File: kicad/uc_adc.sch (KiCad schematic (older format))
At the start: 13 parts, among them IC301 TPD4E001QDBV, IC302 TPD4E001QDBV, IC303 TPD4E001QDBV, IC304 TPD4E001QDBV, IC305 TPD4E001QDBV, IC306 TPD4E001QDBV, U301 TMS320F28388DZWTS

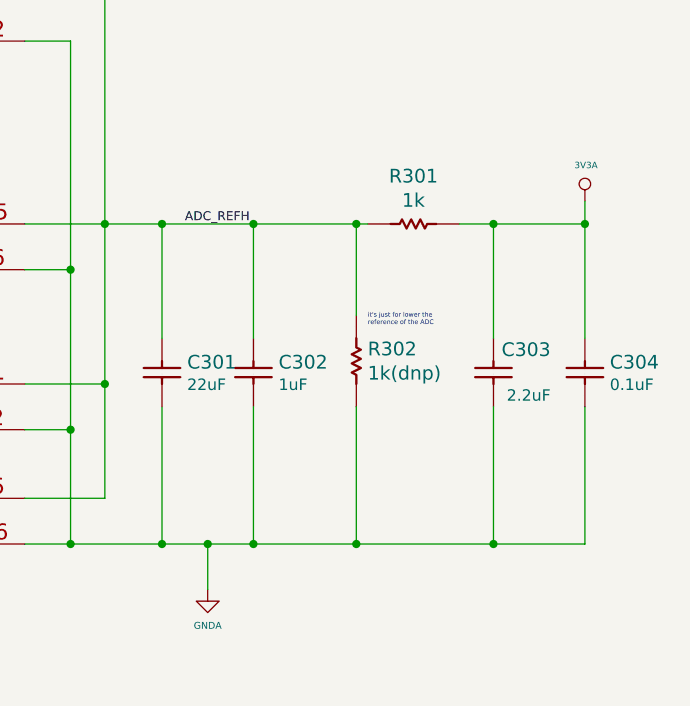
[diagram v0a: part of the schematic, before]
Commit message: bom bom bom...
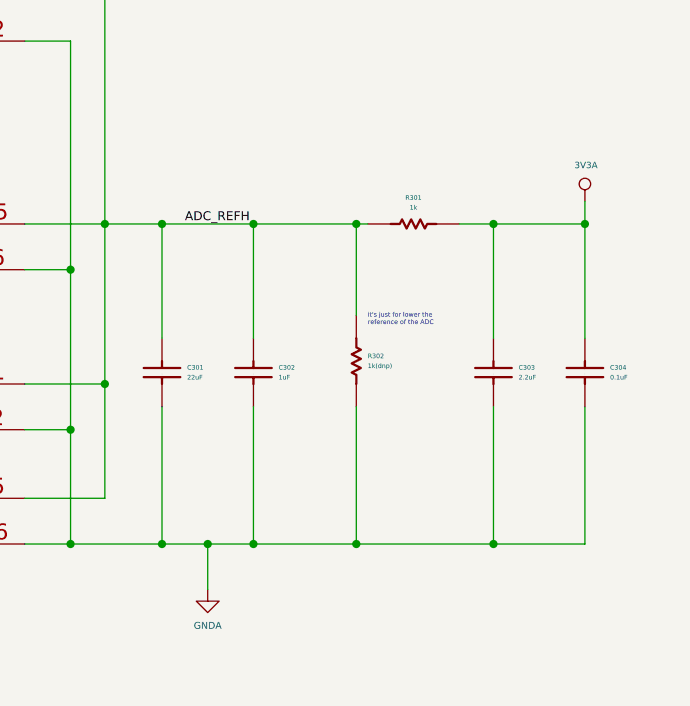
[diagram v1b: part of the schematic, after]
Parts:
- C301: ValueDisplayed 22uF -> (none)
- C302: Description (none) -> CAP CER 1UF 10V X7R 0603; PartNumber (none) -> C0603C105K8RACTU; ValueDisplayed 1uF -> (none); digikey (none) -> 399-11133-1-ND
- C303: ValueDisplayed 2.2uF -> (none)
- C304: Description (none) -> CAP CER 0.1UF 16V X7R 0603; PartNumber (none) -> CC0603KPX7R7BB104; ValueDisplayed 0.1uF -> (none); digikey (none) -> 311-1335-1-ND
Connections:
- net 3V3A: now also R301.2; no longer R301.1
- net ADC_REFH: now also R301.1, R302.1; no longer R301.2, R302.2
- net GNDA: now also R302.2; no longer R302.1
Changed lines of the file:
@@
 	9450 3650 9450 2650
 Wire Wire Line
-	11700 4850 11700 4250
-Wire Wire Line
-	11300 4250 11300 4850
-Wire Wire Line
 	10250 3950 10250 3450
-Wire Wire Line
-	9850 4850 9850 4250
 Connection ~ 9450 4850
 Connection ~ 9450 4350
@@
 U 1 1 5DB391B8
 P 11300 4150
-F 0 "C303" V 11450 4400 60  0000 R CNN
-F 1 "2.2uF" V 11250 4400 50  0000 R CNN
-F 2 "servo:C_0603_1608Metric" H 11300 4150 50  0001 C CNN
-F 3 "" H 11300 4150 50  0001 C CNN
-F 4 "2.2uF" V 800 3250 60  0001 C CNN "ValueDisplayed"
+F 0 "C303" V 11372 4040 20  0000 R CNN
+F 1 "2.2uF" V 11329 4040 20  0000 R CNN
+F 2 "servo:C_0603_1608Metric" H 11300 4050 60  0001 C CNN
+F 3 "" H 11300 4150 60  0000 C CNN
 	1    11300 4150
-	0    1    -1   0
+	0    -1   -1   0
 $EndComp
 $Comp
@@
 U 1 1 5DB391B3
 P 10250 4150
-F 0 "C302" V 10345 4040 60  0000 R CNN
-F 1 "1uF" V 10247 4040 50  0000 R CNN
-F 2 "servo:C_0603_1608Metric" H 10250 4150 50  0001 C CNN
-F 3 "" H 10250 4150 50  0001 C CNN
-F 4 "1uF" V -4150 3450 60  0001 C CNN "ValueDisplayed"
+F 0 "C302" V 10322 4040 20  0000 R CNN
+F 1 "1uF" V 10279 4040 20  0000 R CNN
+F 2 "servo:C_0603_1608Metric" H 10250 4050 60  0001 C CNN
+F 3 "" H 10250 4150 60  0000 C CNN
+F 4 "CAP CER 1UF 10V X7R 0603" H 0   0   50  0001 C CNN "Description"
+F 5 "" H 0   0   50  0001 C CNN "Mfr part number"
+F 6 "399-11133-1-ND" H 0   0   50  0001 C CNN "digikey"
+F 7 "C0603C105K8RACTU" H 0   0   50  0001 C CNN "PartNumber"
 	1    10250 4150
 	0    -1   -1   0
@@
 U 1 1 5DB3916A
 P 9850 4150
-F 0 "C301" V 9945 4040 60  0000 R CNN
-F 1 "22uF" V 9847 4040 50  0000 R CNN
-F 2 "servo:C_0603_1608Metric" H 9850 4150 50  0001 C CNN
-F 3 "" H 9850 4150 50  0001 C CNN
-F 4 "22uF" V 450 -1650 60  0001 C CNN "ValueDisplayed"
+F 0 "C301" V 9922 4040 20  0000 R CNN
+F 1 "22uF" V 9879 4040 20  0000 R CNN
+F 2 "servo:C_0603_1608Metric" H 9850 4050 60  0001 C CNN
+F 3 "" H 9850 4150 60  0000 C CNN
 	1    9850 4150
 	0    -1   -1   0
@@
 U 1 1 5DB39165
 P 11700 4150
-F 0 "C304" V 11795 4259 60  0000 L CNN
-F 1 "0.1uF" V 11697 4259 50  0000 L CNN
-F 2 "servo:C_0603_1608Metric" H 11700 4150 50  0001 C CNN
-F 3 "" H 11700 4150 50  0001 C CNN
-F 4 "0.1uF" V 1600 3250 60  0001 C CNN "ValueDisplayed"
+F 0 "C304" V 11772 4040 20  0000 R CNN
+F 1 "0.1uF" V 11729 4040 20  0000 R CNN
+F 2 "servo:C_0603_1608Metric" H 11700 4050 60  0001 C CNN
+F 3 "" H 11700 4150 60  0000 C CNN
+F 4 "311-1335-1-ND" H 0   0   50  0001 C CNN "digikey"
+F 5 "CAP CER 0.1UF 16V X7R 0603 " H 0   0   50  0001 C CNN "Description"
+F 6 "" H 0   0   50  0001 C CNN "Mfr part number"
+F 7 "CC0603KPX7R7BB104" H 0   0   50  0001 C CNN "PartNumber"
 	1    11700 4150
-	0    1    -1   0
+	0    -1   -1   0
 $EndComp
 $Comp
@@
 U 1 1 5E88CCA6
 P 10950 3450
-F 0 "R301" H 10950 3241 60  0000 C CNN
-F 1 "1k" H 10950 3347 60  0000 C CNN
-F 2 "servo:R_0603_1608Metric" H 10950 3450 50  0001 C CNN
-F 3 "" H 10950 3450 50  0001 C CNN
+F 0 "R301" H 10950 3565 20  0000 C CNN
+F 1 "1k" H 10950 3522 20  0000 C CNN
+F 2 "servo:R_0603_1608Metric" H 10450 3350 60  0001 C CNN
+F 3 "" H 10550 3450 60  0001 C CNN
 F 4 "" V 950 650 60  0001 C CNN "ValueDisplayed"
 	1    10950 3450
-	-1   0    0    1
-$EndComp
-Wire Wire Line
-	10250 4250 10250 4850
+	1    0    0    -1
+$EndComp
 Wire Wire Line
 	9600 3450 9850 3450
@@
 U 1 1 5F076EC8
 P 10700 4050
-F 0 "R302" V 10753 4000 60  0000 R CNN
-F 1 "1k(dnp)" V 10647 4000 60  0000 R CNN
-F 2 "servo:R_0603_1608Metric" H 10700 4050 50  0001 C CNN
-F 3 "" H 10700 4050 50  0001 C CNN
-F 4 "" V 700 1250 60  0001 C CNN "ValueDisplayed"
+F 0 "R302" V 10678 4100 20  0000 L CNN
+F 1 "1k(dnp)" V 10721 4100 20  0000 L CNN
+F 2 "servo:R_0603_1608Metric" H 10200 3950 60  0001 C CNN
+F 3 "" H 10300 4050 60  0001 C CNN
 	1    10700 4050
-	0    -1   -1   0
+	0    1    1    0
 $EndComp
 Wire Wire Line
@@
 Wire Wire Line
 	5550 2450 7050 2450
+Wire Wire Line
+	10250 4250 10250 4850
+Wire Wire Line
+	9850 4250 9850 4850
+Wire Wire Line
+	11300 4250 11300 4850
+Wire Wire Line
+	11700 4250 11700 4850
 $EndSCHEMATC

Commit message: more bom...
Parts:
- C301: Description (none) -> CAP CER 22UF 6.3V X5R 0603; PartNumber (none) -> GRM188R60J226MEA0D; digikey (none) -> 490-7611-1-ND
- C303: Description (none) -> CAP CER 2.2UF 16V X6S 0603; PartNumber (none) -> GRT188C81C225KE13D; digikey (none) -> 490-12287-2-ND
- IC301, IC302, IC303, IC304, IC305, IC306: Description (none) -> TVS DIODE 5.5V 16V SOT23-6; PartNumber (none) -> TPD4E001QDBVRQ1; digikey (none) -> 296-39344-1-ND
- U301: Description (none) -> 32-bit MCU with connectivity manager, 2x C28x+CLA CPU, 1.5 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; price@10 (none) -> 14.96
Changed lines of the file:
@@
 F 2 "servo:C_0603_1608Metric" H 11300 4050 60  0001 C CNN
 F 3 "" H 11300 4150 60  0000 C CNN
+F 4 "CAP CER 2.2UF 16V X6S 0603 " H 0   0   50  0001 C CNN "Description"
+F 5 "GRT188C81C225KE13D" H 0   0   50  0001 C CNN "PartNumber"
+F 6 "490-12287-2-ND" H 0   0   50  0001 C CNN "digikey"
 	1    11300 4150
 	0    -1   -1   0
@@
 F 2 "servo:C_0603_1608Metric" H 9850 4050 60  0001 C CNN
 F 3 "" H 9850 4150 60  0000 C CNN
+F 4 "490-7611-1-ND" H 9850 4150 50  0001 C CNN "digikey"
+F 5 "CAP CER 22UF 6.3V X5R 0603 " H 0   0   50  0001 C CNN "Description"
+F 6 "GRM188R60J226MEA0D" H 0   0   50  0001 C CNN "PartNumber"
 	1    9850 4150
 	0    -1   -1   0
@@
 F 3 "../doc/datasheets/tms320f28388d_datasheet.pdf" H 8150 3750 50  0001 C CNN
 F 4 "TMS320F28388DZWTS" V 1350 -350 60  0001 C CNN "PartNumber"
+F 5 "32-bit MCU with connectivity manager, 2x C28x+CLA CPU, 1.5 MB flash, FPU64, CLB, Ethernet, EtherCAT" H 0   0   50  0001 C CNN "Description"
+F 6 "14.96" H 0   0   50  0001 C CNN "price@10"
 	1    8150 3750
 	1    0    0    -1
@@
 F 2 "servo:SOT-23-6" H 2700 1850 60  0001 C CNN
 F 3 "../doc/datasheets/tpd4e001-q1.pdf" H 2750 2150 60  0001 C CNN
+F 4 "TVS DIODE 5.5V 16V SOT23-6 " H 0   0   50  0001 C CNN "Description"
+F 5 "TPD4E001QDBVRQ1" H 0   0   50  0001 C CNN "PartNumber"
+F 6 " 296-39344-1-ND" H 0   0   50  0001 C CNN "digikey"
 	1    2700 1850
 	0    -1   -1   0
@@
 F 2 "servo:SOT-23-6" H 3300 1850 60  0001 C CNN
 F 3 "../doc/datasheets/tpd4e001-q1.pdf" H 3350 2150 60  0001 C CNN
+F 4 "TVS DIODE 5.5V 16V SOT23-6 " H 0   0   50  0001 C CNN "Description"
+F 5 "TPD4E001QDBVRQ1" H 0   0   50  0001 C CNN "PartNumber"
+F 6 " 296-39344-1-ND" H 0   0   50  0001 C CNN "digikey"
 	1    3300 1850
 	0    1    -1   0
@@
 F 2 "servo:SOT-23-6" H 3900 1850 60  0001 C CNN
 F 3 "../doc/datasheets/tpd4e001-q1.pdf" H 3950 2150 60  0001 C CNN
+F 4 "TVS DIODE 5.5V 16V SOT23-6 " H 0   0   50  0001 C CNN "Description"
+F 5 "TPD4E001QDBVRQ1" H 0   0   50  0001 C CNN "PartNumber"
+F 6 " 296-39344-1-ND" H 0   0   50  0001 C CNN "digikey"
 	1    3900 1850
 	0    -1   -1   0
@@
 F 2 "servo:SOT-23-6" H 5200 1850 60  0001 C CNN
 F 3 "../doc/datasheets/tpd4e001-q1.pdf" H 5250 2150 60  0001 C CNN
+F 4 "TVS DIODE 5.5V 16V SOT23-6 " H 0   0   50  0001 C CNN "Description"
+F 5 "TPD4E001QDBVRQ1" H 0   0   50  0001 C CNN "PartNumber"
+F 6 " 296-39344-1-ND" H 0   0   50  0001 C CNN "digikey"
 	1    5200 1850
 	0    -1   -1   0
@@
 F 2 "servo:SOT-23-6" H 4500 1850 60  0001 C CNN
 F 3 "../doc/datasheets/tpd4e001-q1.pdf" H 4550 2150 60  0001 C CNN
+F 4 "TVS DIODE 5.5V 16V SOT23-6 " H 0   0   50  0001 C CNN "Description"
+F 5 "TPD4E001QDBVRQ1" H 0   0   50  0001 C CNN "PartNumber"
+F 6 " 296-39344-1-ND" H 0   0   50  0001 C CNN "digikey"
 	1    4500 1850
 	0    -1   -1   0
@@
 F 2 "servo:SOT-23-6" H 5800 1850 60  0001 C CNN
 F 3 "../doc/datasheets/tpd4e001-q1.pdf" H 5850 2150 60  0001 C CNN
+F 4 "TVS DIODE 5.5V 16V SOT23-6 " H 0   0   50  0001 C CNN "Description"
+F 5 "TPD4E001QDBVRQ1" H 0   0   50  0001 C CNN "PartNumber"
+F 6 " 296-39344-1-ND" H 0   0   50  0001 C CNN "digikey"
 	1    5800 1850
 	0    1    -1   0

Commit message: stackup
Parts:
- C301: price@10 (none) -> 0.19400
- C302: price@10 (none) -> 0.06400
- C303: digikey 490-12287-2-ND -> 490-12287-1-ND; price@10 (none) -> 0.35500
- C304: price@10 (none) -> 0.05800
- IC301, IC302, IC303, IC304, IC305, IC306: digikey 296-39344-1-ND -> 296-39344-1-ND; price@10 (none) -> 0.56800
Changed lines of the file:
@@
 F 4 "CAP CER 2.2UF 16V X6S 0603 " H 0   0   50  0001 C CNN "Description"
 F 5 "GRT188C81C225KE13D" H 0   0   50  0001 C CNN "PartNumber"
-F 6 "490-12287-2-ND" H 0   0   50  0001 C CNN "digikey"
+F 6 "490-12287-1-ND" H 0   0   50  0001 C CNN "digikey"
+F 7 "0.35500" H 0   0   50  0001 C CNN "price@10"
 	1    11300 4150
 	0    -1   -1   0
@@
 F 3 "" H 10250 4150 60  0000 C CNN
 F 4 "CAP CER 1UF 10V X7R 0603" H 0   0   50  0001 C CNN "Description"
-F 5 "" H 0   0   50  0001 C CNN "Mfr part number"
-F 6 "399-11133-1-ND" H 0   0   50  0001 C CNN "digikey"
-F 7 "C0603C105K8RACTU" H 0   0   50  0001 C CNN "PartNumber"
+F 5 "399-11133-1-ND" H 0   0   50  0001 C CNN "digikey"
+F 6 "C0603C105K8RACTU" H 0   0   50  0001 C CNN "PartNumber"
+F 7 "0.06400" H 0   0   50  0001 C CNN "price@10"
 	1    10250 4150
 	0    -1   -1   0
@@
 F 5 "CAP CER 22UF 6.3V X5R 0603 " H 0   0   50  0001 C CNN "Description"
 F 6 "GRM188R60J226MEA0D" H 0   0   50  0001 C CNN "PartNumber"
+F 7 "0.19400" H 0   0   50  0001 C CNN "price@10"
 	1    9850 4150
 	0    -1   -1   0
@@
 F 4 "311-1335-1-ND" H 0   0   50  0001 C CNN "digikey"
 F 5 "CAP CER 0.1UF 16V X7R 0603 " H 0   0   50  0001 C CNN "Description"
-F 6 "" H 0   0   50  0001 C CNN "Mfr part number"
-F 7 "CC0603KPX7R7BB104" H 0   0   50  0001 C CNN "PartNumber"
+F 6 "CC0603KPX7R7BB104" H 0   0   50  0001 C CNN "PartNumber"
+F 7 "0.05800" H 0   0   50  0001 C CNN "price@10"
 	1    11700 4150
 	0    -1   -1   0
@@
 F 2 "servo:R_0603_1608Metric" H 10450 3350 60  0001 C CNN
 F 3 "" H 10550 3450 60  0001 C CNN
-F 4 "" V 950 650 60  0001 C CNN "ValueDisplayed"
 	1    10950 3450
 	1    0    0    -1
@@
 F 4 "TVS DIODE 5.5V 16V SOT23-6 " H 0   0   50  0001 C CNN "Description"
 F 5 "TPD4E001QDBVRQ1" H 0   0   50  0001 C CNN "PartNumber"
-F 6 " 296-39344-1-ND" H 0   0   50  0001 C CNN "digikey"
+F 6 "296-39344-1-ND" H 0   0   50  0001 C CNN "digikey"
+F 7 "0.56800" H 0   0   50  0001 C CNN "price@10"
 	1    2700 1850
 	0    -1   -1   0
@@
 F 4 "TVS DIODE 5.5V 16V SOT23-6 " H 0   0   50  0001 C CNN "Description"
 F 5 "TPD4E001QDBVRQ1" H 0   0   50  0001 C CNN "PartNumber"
-F 6 " 296-39344-1-ND" H 0   0   50  0001 C CNN "digikey"
+F 6 "296-39344-1-ND" H 0   0   50  0001 C CNN "digikey"
+F 7 "0.56800" H 0   0   50  0001 C CNN "price@10"
 	1    3300 1850
 	0    1    -1   0
@@
 F 4 "TVS DIODE 5.5V 16V SOT23-6 " H 0   0   50  0001 C CNN "Description"
 F 5 "TPD4E001QDBVRQ1" H 0   0   50  0001 C CNN "PartNumber"
-F 6 " 296-39344-1-ND" H 0   0   50  0001 C CNN "digikey"
+F 6 "296-39344-1-ND" H 0   0   50  0001 C CNN "digikey"
+F 7 "0.56800" H 0   0   50  0001 C CNN "price@10"
 	1    3900 1850
 	0    -1   -1   0
@@
 F 4 "TVS DIODE 5.5V 16V SOT23-6 " H 0   0   50  0001 C CNN "Description"
 F 5 "TPD4E001QDBVRQ1" H 0   0   50  0001 C CNN "PartNumber"
-F 6 " 296-39344-1-ND" H 0   0   50  0001 C CNN "digikey"
+F 6 "296-39344-1-ND" H 0   0   50  0001 C CNN "digikey"
+F 7 "0.56800" H 0   0   50  0001 C CNN "price@10"
 	1    5200 1850
 	0    -1   -1   0
@@
 F 4 "TVS DIODE 5.5V 16V SOT23-6 " H 0   0   50  0001 C CNN "Description"
 F 5 "TPD4E001QDBVRQ1" H 0   0   50  0001 C CNN "PartNumber"
-F 6 " 296-39344-1-ND" H 0   0   50  0001 C CNN "digikey"
+F 6 "296-39344-1-ND" H 0   0   50  0001 C CNN "digikey"
+F 7 "0.56800" H 0   0   50  0001 C CNN "price@10"
 	1    4500 1850
 	0    -1   -1   0
@@
 F 4 "TVS DIODE 5.5V 16V SOT23-6 " H 0   0   50  0001 C CNN "Description"
 F 5 "TPD4E001QDBVRQ1" H 0   0   50  0001 C CNN "PartNumber"
-F 6 " 296-39344-1-ND" H 0   0   50  0001 C CNN "digikey"
+F 6 "296-39344-1-ND" H 0   0   50  0001 C CNN "digikey"
+F 7 "0.56800" H 0   0   50  0001 C CNN "price@10"
 	1    5800 1850
 	0    1    -1   0

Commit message: bom copleted
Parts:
- R301, R302: Description (none) -> 1 kOhms ±5% 0.1W, 1/10W Chip Resistor 0603 (1608 Metric) Mo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; PartNumber (none) -> RC0603JR-071KL; digikey (none) -> 311-1.0KGRCT-ND; price@10 (none) -> 0.01900
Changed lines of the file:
@@
 F 2 "servo:R_0603_1608Metric" H 10450 3350 60  0001 C CNN
 F 3 "" H 10550 3450 60  0001 C CNN
+F 4 "1 kOhms ±5% 0.1W, 1/10W Chip Resistor 0603 (1608 Metric) Moisture Resistant Thick Film " H 0   0   50  0001 C CNN "Description"
+F 5 "RC0603JR-071KL" H 0   0   50  0001 C CNN "PartNumber"
+F 6 "311-1.0KGRCT-ND" H 0   0   50  0001 C CNN "digikey"
+F 7 "0.01900" H 0   0   50  0001 C CNN "price@10"
 	1    10950 3450
 	1    0    0    -1
@@
 F 2 "servo:R_0603_1608Metric" H 10200 3950 60  0001 C CNN
 F 3 "" H 10300 4050 60  0001 C CNN
+F 4 "1 kOhms ±5% 0.1W, 1/10W Chip Resistor 0603 (1608 Metric) Moisture Resistant Thick Film " H 0   0   50  0001 C CNN "Description"
+F 5 "RC0603JR-071KL" H 0   0   50  0001 C CNN "PartNumber"
+F 6 "311-1.0KGRCT-ND" H 0   0   50  0001 C CNN "digikey"
+F 7 "0.01900" H 0   0   50  0001 C CNN "price@10"
 	1    10700 4050
 	0    1    1    0
